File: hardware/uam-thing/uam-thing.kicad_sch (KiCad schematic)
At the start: 2 parts, among them J1 ESP_Left, J2 ESP_Right

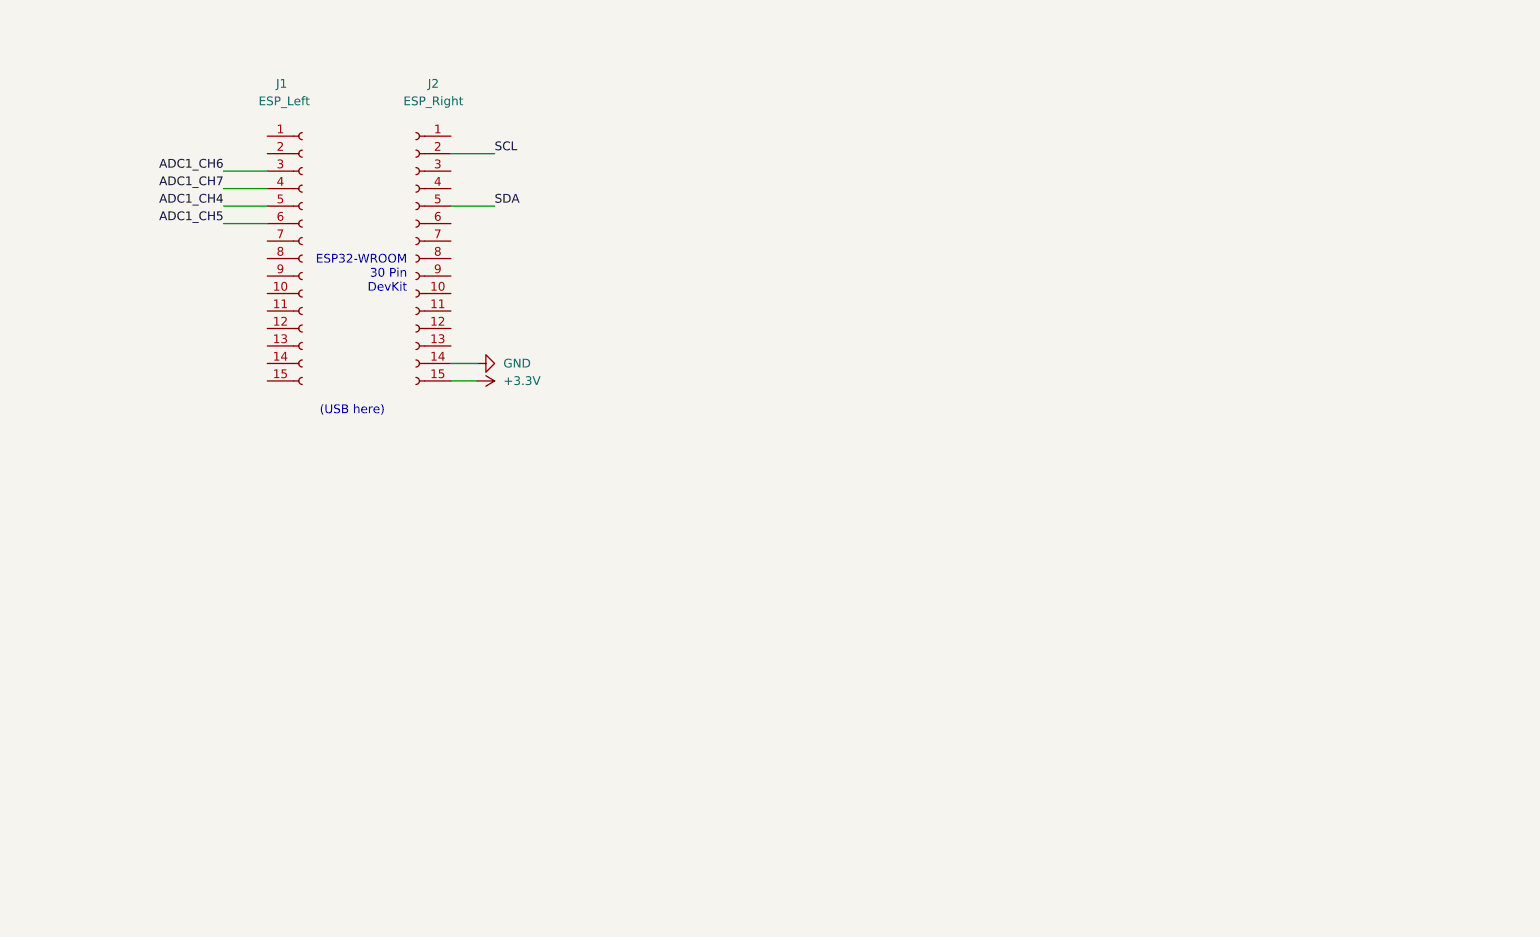
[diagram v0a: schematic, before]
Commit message: First version of hardware design
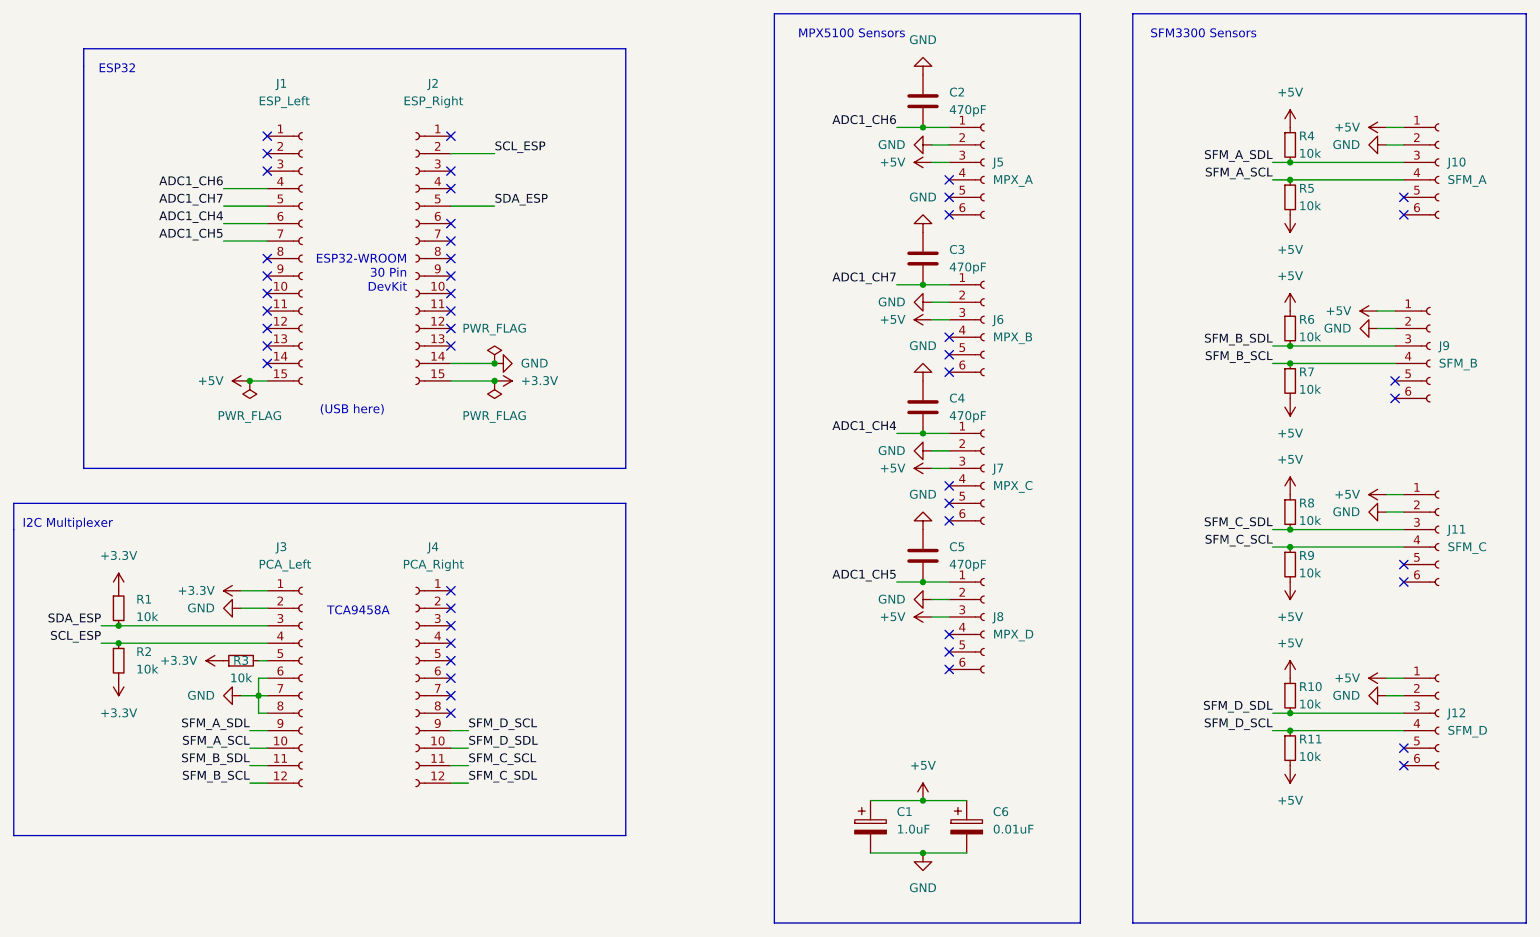
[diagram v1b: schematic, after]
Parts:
- added C1: 1.0uF, Capacitor_THT:CP_Radial_D5.0mm_P2.00mm, symbol Device:C_Polarized
- added C2, C3, C4, C5: 470pF, Capacitor_THT:C_Disc_D4.7mm_W2.5mm_P5.00mm, symbol Device:C
- added C6: 0.01uF, Capacitor_THT:C_Disc_D4.7mm_W2.5mm_P5.00mm, symbol Device:C_Polarized
- added J10: SFM_A, Connector_JST:JST_XH_B6B-XH-A_1x06_P2.50mm_Vertical, symbol Connector:Conn_01x06_Female
- added J11: SFM_C, Connector_JST:JST_XH_B6B-XH-A_1x06_P2.50mm_Vertical, symbol Connector:Conn_01x06_Female
- added J12: SFM_D, Connector_JST:JST_XH_B6B-XH-A_1x06_P2.50mm_Vertical, symbol Connector:Conn_01x06_Female
- added J3: PCA_Left, symbol Connector:Conn_01x12_Female
- added J4: PCA_Right, symbol Connector:Conn_01x12_Female
- added J5: MPX_A, symbol Connector:Conn_01x06_Female
- added J6: MPX_B, symbol Connector:Conn_01x06_Female
- added J7: MPX_C, Connector_PinHeader_2.54mm:PinHeader_1x06_P2.54mm_Vertical, symbol Connector:Conn_01x06_Female
- added J8: MPX_D, Connector_PinHeader_2.54mm:PinHeader_1x06_P2.54mm_Vertical, symbol Connector:Conn_01x06_Female
- added J9: SFM_B, Connector_JST:JST_XH_B6B-XH-A_1x06_P2.50mm_Vertical, symbol Connector:Conn_01x06_Female
- added R1, R10, R11, R2, R3, R4, R5, R6, R7, R8, R9: 10k, Resistor_THT:R_Axial_DIN0207_L6.3mm_D2.5mm_P10.16mm_Horizontal, symbol Device:R_Small
- J1, J2: footprint (none) -> Connector_PinHeader_2.54mm:PinHeader_1x15_P2.54mm_Vertical
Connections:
- net +3.3V: now also J3.1 (Pin_1), R1.1, R2.2, R3.1
- net ADC1_CH4: now also J1.6 (Pin_6), C4.2, J7.1 (Pin_1); no longer J1.5 (Pin_5)
- net ADC1_CH5: now also J1.7 (Pin_7), C5.2, J8.1 (Pin_1); no longer J1.6 (Pin_6)
- net ADC1_CH6: now also J1.4 (Pin_4), C2.2, J5.1 (Pin_1); no longer J1.3 (Pin_3)
- net ADC1_CH7: now also J1.5 (Pin_5), C3.2, J6.1 (Pin_1); no longer J1.4 (Pin_4)
- net GND: now also C1.2, C2.1, C3.1, C4.1, C5.1, C6.2, J10.2 (Pin_2), J11.2 (Pin_2), J12.2 (Pin_2), J3.2 (Pin_2), J3.6 (Pin_6), J3.7 (Pin_7), J3.8 (Pin_8), J5.2 (Pin_2), J6.2 (Pin_2), J7.2 (Pin_2), J8.2 (Pin_2), J9.2 (Pin_2)
- net +5V: now reaches J1.15 (Pin_15)
- net +5V: now also C1.1, C6.1, J10.1 (Pin_1), J11.1 (Pin_1), J12.1 (Pin_1), J5.3 (Pin_3), J6.3 (Pin_3), J7.3 (Pin_3), J8.3 (Pin_3), J9.1 (Pin_1), R10.1, R11.2, R4.1, R5.2, R6.1, R7.2, R8.1, R9.2
- net SCL renamed SCL_ESP
- net SCL_ESP: now also J3.4 (Pin_4), R2.1
- net SDA renamed SDA_ESP
- net SDA_ESP: now also J3.3 (Pin_3), R1.2
- new net: J3.5 (Pin_5), R3.2
- new net SFM_A_SCL: J10.4 (Pin_4), J3.10 (Pin_10), R5.1
- new net SFM_A_SDL: J10.3 (Pin_3), J3.9 (Pin_9), R4.2
- new net SFM_B_SCL: J3.12 (Pin_12), J9.4 (Pin_4), R7.1
- new net SFM_B_SDL: J3.11 (Pin_11), J9.3 (Pin_3), R6.2
- new net SFM_C_SCL: J11.4 (Pin_4), J4.11 (Pin_11), R9.1
- new net SFM_C_SDL: J11.3 (Pin_3), J4.12 (Pin_12), R8.2
- new net SFM_D_SCL: J12.4 (Pin_4), J4.9 (Pin_9), R11.1
- new net SFM_D_SDL: J12.3 (Pin_3), J4.10 (Pin_10), R10.2
- no-connect marks 0 -> 49
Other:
- note added: "ESP32"
- note added: "I2C Multiplexer"
- note added: "MPX5100 Sensors"
- note added: "SFM3300 Sensors"
- note added: "TCA9458A"
